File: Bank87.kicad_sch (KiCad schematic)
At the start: 1 part, among them U1 XCKU5P-FFVB676

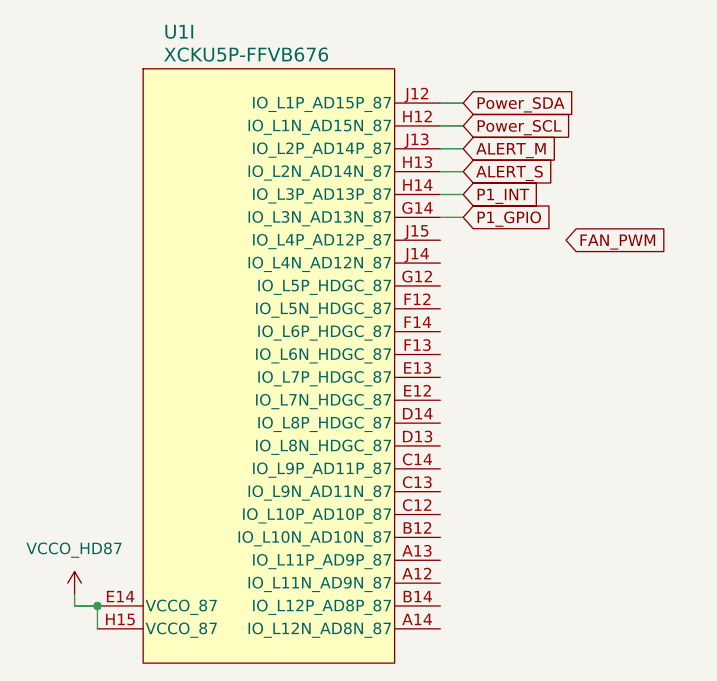
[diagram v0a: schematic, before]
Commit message: finishing schematic
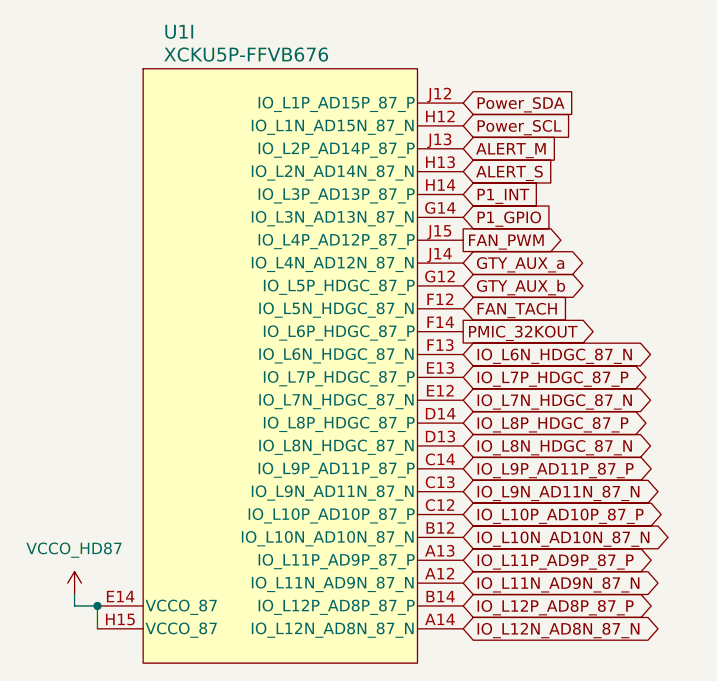
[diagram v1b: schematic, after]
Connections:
- net FAN_PWM: now also U1.J15 (IO_L4P_AD12P_87_P)
- net IO_L11N_AD9N_87_N: now reaches U1.A12 (IO_L11N_AD9N_87_N)
- net IO_L11P_AD9P_87_P: now reaches U1.A13 (IO_L11P_AD9P_87_P)
- net IO_L12N_AD8N_87_N: now reaches U1.A14 (IO_L12N_AD8N_87_N)
- net IO_L10N_AD10N_87_N: now reaches U1.B12 (IO_L10N_AD10N_87_N)
- net IO_L12P_AD8P_87_P: now reaches U1.B14 (IO_L12P_AD8P_87_P)
- net IO_L10P_AD10P_87_P: now reaches U1.C12 (IO_L10P_AD10P_87_P)
- net IO_L9N_AD11N_87_N: now reaches U1.C13 (IO_L9N_AD11N_87_N)
- net IO_L9P_AD11P_87_P: now reaches U1.C14 (IO_L9P_AD11P_87_P)
- net IO_L8N_HDGC_87_N: now reaches U1.D13 (IO_L8N_HDGC_87_N)
- net IO_L8P_HDGC_87_P: now reaches U1.D14 (IO_L8P_HDGC_87_P)
- net IO_L7N_HDGC_87_N: now reaches U1.E12 (IO_L7N_HDGC_87_N)
- net IO_L7P_HDGC_87_P: now reaches U1.E13 (IO_L7P_HDGC_87_P)
- net FAN_TACH: now reaches U1.F12 (IO_L5N_HDGC_87_N)
- net IO_L6N_HDGC_87_N: now reaches U1.F13 (IO_L6N_HDGC_87_N)
- net PMIC_32KOUT: now reaches U1.F14 (IO_L6P_HDGC_87_P)
- net GTY_AUX_b: now reaches U1.G12 (IO_L5P_HDGC_87_P)
- net GTY_AUX_a: now reaches U1.J14 (IO_L4N_AD12N_87_N)
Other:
- moved on the sheet: U1I
